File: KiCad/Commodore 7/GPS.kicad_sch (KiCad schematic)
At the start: 1 part, among them U2 NEO-M9N-00B

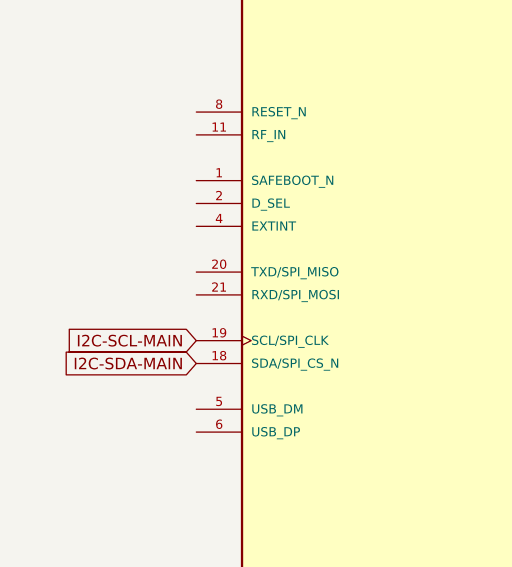
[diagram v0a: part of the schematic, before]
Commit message: helloooo
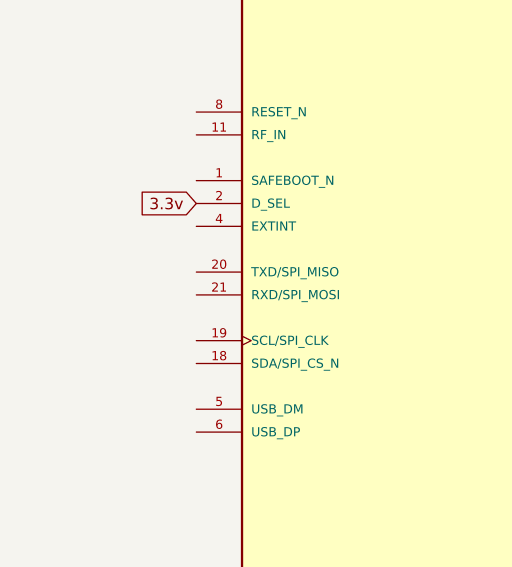
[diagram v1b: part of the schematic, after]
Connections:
- net 3.3v: now also U2.2 (D_SEL)
- net I2C-SCL-MAIN: no longer names the net of U2.19 (SCL/SPI_CLK)
- net I2C-SDA-MAIN: no longer names the net of U2.18 (SDA/SPI_CS_N)
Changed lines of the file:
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@@
+	(global_label "3.3v"
+		(shape input)
+		(at 95.25 85.09 180)
+		(fields_autoplaced yes)
+		(effects
+			(font
+				(size 1.27 1.27)
+			)
+			(justify right)
+		)
+		(property "Intersheetrefs" "${INTERSHEET_REFS}"
+			(at 88.2734 85.09 0)
+			(effects
+				(font
+					(size 1.27 1.27)
+				)
+				(justify right)
+				(hide yes)
+			)
+		)
+	)
 	(global_label "3.3v"
 		(shape input)
@@
 				(hide yes)
 			)
-		)
-	)
-	(global_label "I2C-SCL-MAIN"
-		(shape input)
-		(at 95.25 100.33 180)
-		(fields_autoplaced yes)
-		(effects
-			(font
-				(size 1.27 1.27)
-			)
-			(justify right)
-		)
-		(property "Intersheetrefs" "${INTERSHEET_REFS}"
-			(at 78.0528 100.33 0)
-			(effects
-				(font
-					(size 1.27 1.27)
-				)
-				(justify right)
-				(hide yes)
-			)
-		)
-	)
-	(global_label "I2C-SDA-MAIN"
-		(shape input)
-		(at 95.25 102.87 180)
-		(fields_autoplaced yes)
-		(effects
-			(font
-				(size 1.27 1.27)
-			)
-			(justify right)
-		)
-		(property "Intersheetrefs" "${INTERSHEET_REFS}"
-			(at 77.9923 102.87 0)
-			(effects
-				(font
-					(size 1.27 1.27)
-				)
-				(justify right)
-				(hide yes)
-			)

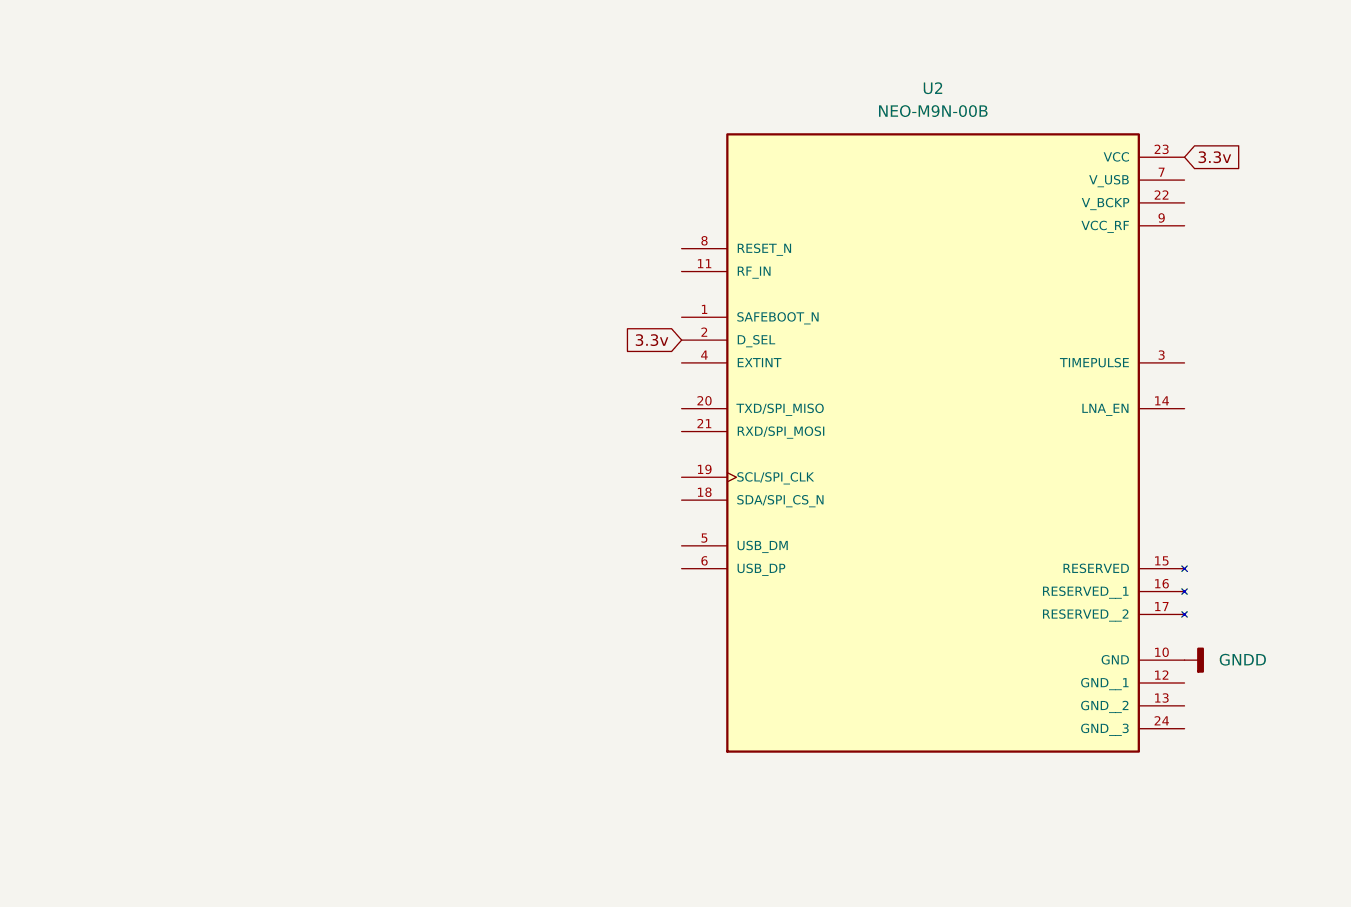
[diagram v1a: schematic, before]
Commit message: hi
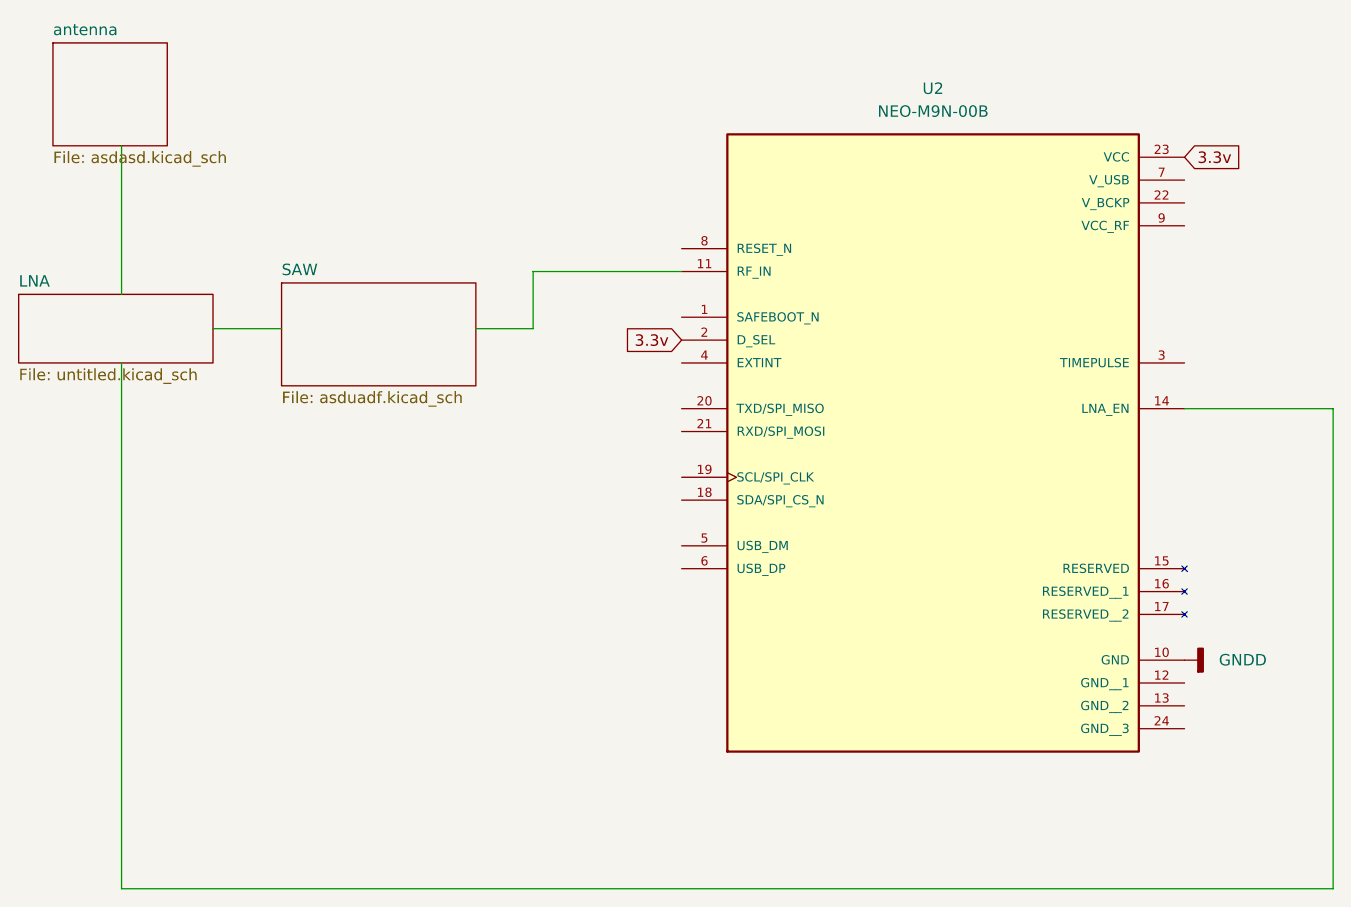
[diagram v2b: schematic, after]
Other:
- added sheet LNA (untitled.kicad_sch)
- added sheet SAW (asduadf.kicad_sch)
- added sheet antenna (asdasd.kicad_sch)
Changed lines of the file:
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@@
 	(generator_version "9.0")
 	(paper "A4")
+	(wire
+		(pts
+			(xy 33.02 146.05) (xy 167.64 146.05)
+		)
+		(stroke
+			(width 0)
+			(type default)
+		)
+	)
+	(wire
+		(pts
+			(xy 167.64 92.71) (xy 151.13 92.71)
+		)
+		(stroke
+			(width 0)
+			(type default)
+		)
+	)
+	(wire
+		(pts
+			(xy 72.39 83.82) (xy 78.74 83.82)
+		)
+		(stroke
+			(width 0)
+			(type default)
+		)
+	)
+	(wire
+		(pts
+			(xy 43.18 83.82) (xy 50.8 83.82)
+		)
+		(stroke
+			(width 0)
+			(type default)
+		)
+	)
+	(wire
+		(pts
+			(xy 95.25 77.47) (xy 78.74 77.47)
+		)
+		(stroke
+			(width 0)
+			(type default)
+		)
+	)
+	(wire
+		(pts
+			(xy 167.64 146.05) (xy 167.64 92.71)
+		)
+		(stroke
+			(width 0)
+			(type default)
+		)
+	)
+	(wire
+		(pts
+			(xy 33.02 87.63) (xy 33.02 146.05)
+		)
+		(stroke
+			(width 0)
+			(type default)
+		)
+	)
+	(wire
+		(pts
+			(xy 33.02 63.5) (xy 33.02 80.01)
+		)
+		(stroke
+			(width 0)
+			(type default)
+		)
+	)
+	(wire
+		(pts
+			(xy 78.74 77.47) (xy 78.74 83.82)
+		)
+		(stroke
+			(width 0)
+			(type default)
+		)
+	)
 	(global_label "3.3v"
 		(shape input)
@@
 				)
 			)
+		)
+	)
+	(sheet
+		(at 25.4 52.07)
+		(size 12.7 11.43)
+		(exclude_from_sim no)
+		(in_bom yes)
+		(on_board yes)
+		(dnp no)
+		(fields_autoplaced yes)
+		(stroke
+			(width 0.1524)
+			(type solid)
+		)
+		(fill
+			(color 0 0 0 0.0000)
+		)
+		(property "Sheetname" "antenna"
+			(at 25.4 51.3584 0)
+			(effects
+				(font
+					(size 1.27 1.27)
+				)
+				(justify left bottom)
+			)
+		)
+		(property "Sheetfile" "asdasd.kicad_sch"
+			(at 25.4 64.0846 0)
+			(effects
+				(font
+					(size 1.27 1.27)
+				)
+				(justify left top)
+			)
+		)
+		(instances
+			(project "Commodore 7"
+				(path "/42cf917d-ec14-4557-b98d-6a3f3b8cf25c/bd54c1aa-247c-4340-9de9-44d0c0e040e9"
+					(page "12")
+				)
+			)
+		)
+	)
+	(sheet
+		(at 50.8 78.74)
+		(size 21.59 11.43)
+		(exclude_from_sim no)
+		(in_bom yes)
+		(on_board yes)
+		(dnp no)
+		(fields_autoplaced yes)
+		(stroke
+			(width 0.1524)
+			(type solid)
+		)
+		(fill
+			(color 0 0 0 0.0000)
+		)
+		(property "Sheetname" "SAW"
+			(at 50.8 78.0284 0)
+			(effects
+				(font
+					(size 1.27 1.27)
+				)
+				(justify left bottom)
+			)
+		)
+		(property "Sheetfile" "asduadf.kicad_sch"
+			(at 50.8 90.7546 0)
+			(effects
+				(font
+					(size 1.27 1.27)
+				)
+				(justify left top)
+			)
+		)
+		(instances
+			(project "Commodore 7"
+				(path "/42cf917d-ec14-4557-b98d-6a3f3b8cf25c/bd54c1aa-247c-4340-9de9-44d0c0e040e9"
+					(page "11")
+				)
+			)
+		)
+	)
+	(sheet
+		(at 21.59 80.01)
+		(size 21.59 7.62)
+		(exclude_from_sim no)
+		(in_bom yes)
+		(on_board yes)
+		(dnp no)
+		(fields_autoplaced yes)
+		(stroke
+			(width 0.1524)
+			(type solid)
+		)
+		(fill
+			(color 0 0 0 0.0000)
+		)
+		(property "Sheetname" "LNA"
+			(at 21.59 79.2984 0)
+			(effects
+				(font
+					(size 1.27 1.27)
+				)
+				(justify left bottom)
+			)
+		)
+		(property "Sheetfile" "untitled.kicad_sch"
+			(at 21.59 88.2146 0)
+			(effects
+				(font
+					(size 1.27 1.27)
+				)
+				(justify left top)
+			)
+		)
+		(instances
+			(project "Commodore 7"
+				(path "/42cf917d-ec14-4557-b98d-6a3f3b8cf25c/bd54c1aa-247c-4340-9de9-44d0c0e040e9"
+					(page "10")
+				)
+			)
